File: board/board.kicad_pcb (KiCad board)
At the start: 4 copper layers, 29 x 29 mm, 32 parts, among them J1 001_I2C, J2 011_GPIO, Q1 Q_PMOS_DGS, Q2 Q_NMOS_DGS, U1 ALED7709ATR

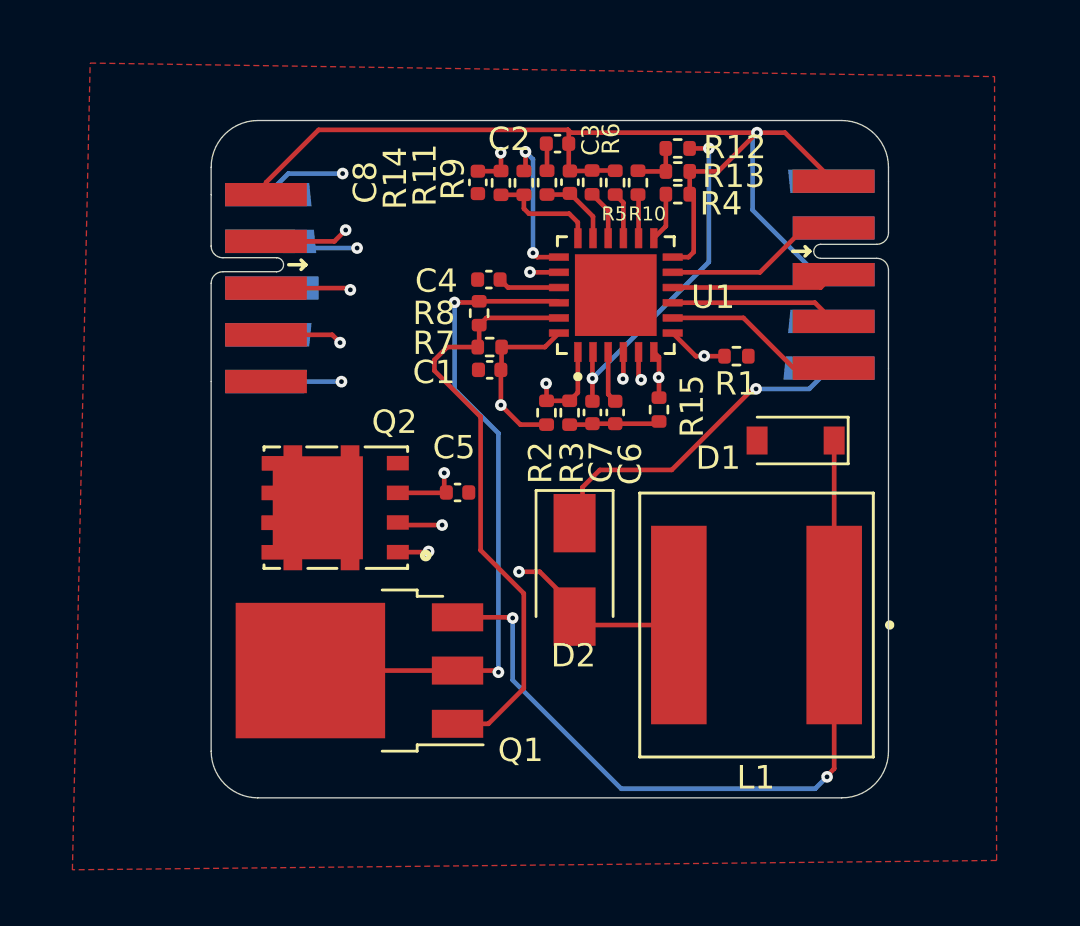
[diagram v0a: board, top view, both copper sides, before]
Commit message: Update PCB
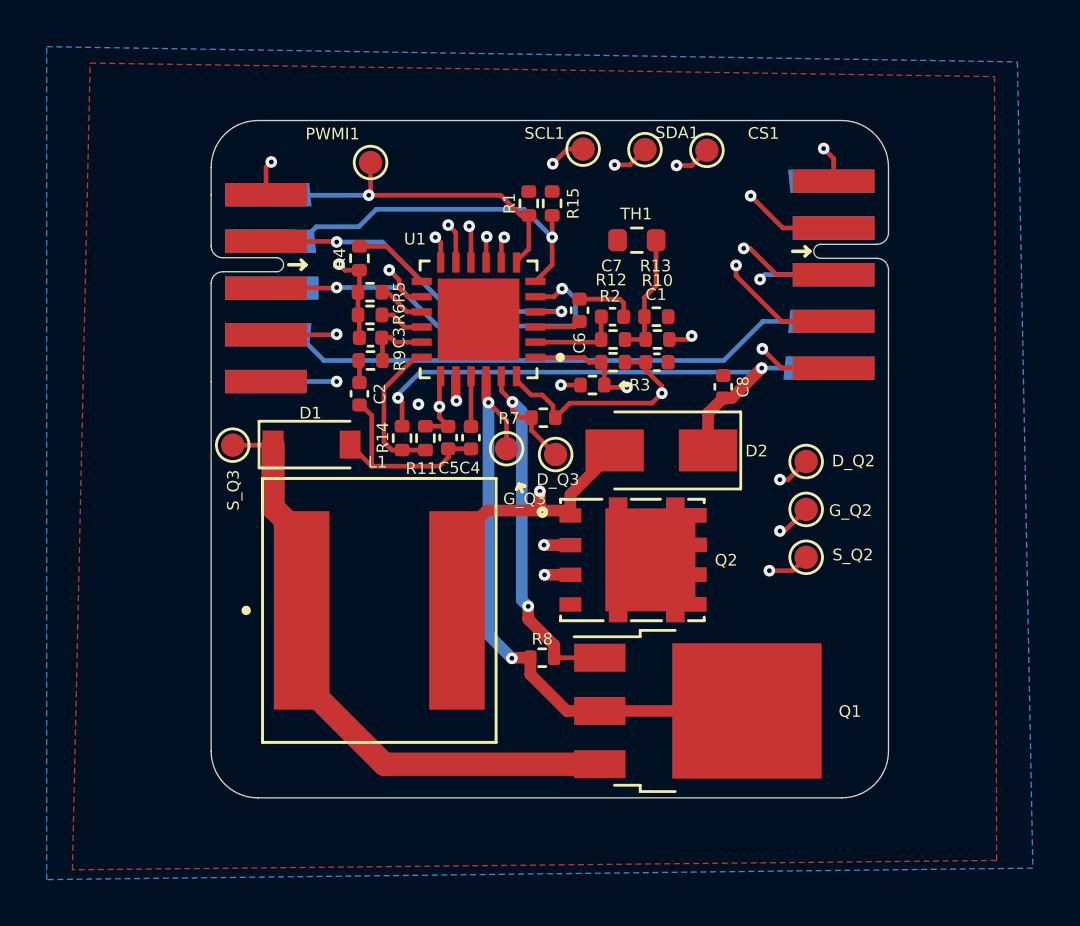
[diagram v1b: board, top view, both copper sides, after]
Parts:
- added CS1: TestPoint, TestPoint:TestPoint_Pad_D1.0mm, F.Cu at (161.2, 91.3)
- added D_Q2: TestPoint, TestPoint:TestPoint_Pad_D1.0mm, F.Cu at (165.5, 104.6)
- added D_Q3: TestPoint, TestPoint:TestPoint_Pad_D1.0mm, F.Cu at (154.8, 104.3)
- added G_Q2: TestPoint, TestPoint:TestPoint_Pad_D1.0mm, F.Cu at (165.5, 106.7)
- added G_Q3: TestPoint, TestPoint:TestPoint_Pad_D1.0mm, F.Cu at (152.7, 104.0)
- added PWMI1: TestPoint, TestPoint:TestPoint_Pad_D1.0mm, F.Cu at (146.8, 91.8)
- added SCL1: TestPoint, TestPoint:TestPoint_Pad_D1.0mm, F.Cu at (155.9, 91.2)
- added SDA1: TestPoint, TestPoint:TestPoint_Pad_D1.0mm, F.Cu at (158.6, 91.2)
- added S_Q2: TestPoint, TestPoint:TestPoint_Pad_D1.0mm, F.Cu at (165.5, 108.7)
- added S_Q3: TestPoint, TestPoint:TestPoint_Pad_D1.0mm, F.Cu at (140.9, 103.9)
- added TH1: 10kΩ, Resistor_SMD:R_0603_1608Metric, F.Cu at (158.2, 95.1)
- C1, C8: value C_Small -> 10uF
- C4, C6, C7: value C_Small -> 1uF
- L1: value L -> 15uH
- R10: value R_Small -> 2kΩ
- R12: value R_Small -> 1,8kΩ
- R13: value R_Small -> 1.1kΩ
- R4: value R_Small -> 6,8kΩ
- R5: value R_Small -> 62kΩ
- R7: value R_Small -> 39 mΩ
- moved D1 20.7 mm to (144.3, 103.9), turned to 0 degrees
- moved L1 16.2 mm to (147.2, 111.0), turned to 0 degrees
- moved R8 15.0 mm to (154.2, 113.0), turned to 0 degrees
- moved Q1 14.6 mm to (160.8, 115.3), turned to 0 degrees
- moved R4 13.9 mm to (146.3, 95.9), turned to 90 degrees
- moved C8 13.7 mm to (161.9, 101.4), turned to 90 degrees
- moved C2 13.7 mm to (146.3, 101.7), turned to -90 degrees
- moved Q2 12.9 mm to (158.0, 108.8), turned to 0 degrees
- moved R14 11.7 mm to (148.2, 103.6)
- moved R11 11.7 mm to (149.2, 103.6)
- moved R5 11.5 mm to (146.8, 97.3), turned to 0 degrees
- moved R6 11.1 mm to (146.8, 98.3), turned to 0 degrees
- moved R1 11.0 mm to (153.6, 93.5), turned to -90 degrees
- moved C3 10.8 mm to (146.8, 99.3), turned to 180 degrees
- moved R9 10.7 mm to (146.8, 100.3), turned to 0 degrees
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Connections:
- J1 pad 9: unconnected-(J1-3.3V-Pad9) -> 3.3V
- J2 pad 9: unconnected-(J2-3.3V-Pad9) -> 3.3V
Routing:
- net GND: track 50.4 -> 23.8 mm, vias 1 -> 7
- net 3.3V: track 0.00 -> 25.3 mm
- net /implementation/PWMI: track 34.5 -> 15.2 mm, vias 2 -> 1
- net /implementation/Enable: track 17.0 -> 33.3 mm, vias 2 -> 3
- net Net-(U1-TSNS): track 1.88 -> 18.0 mm, vias 0 -> 2
- net /implementation/common_Anode: track 37.8 -> 25.1 mm
- net /implementation/CH4: track 7.68 -> 19.9 mm, vias 0 -> 2
- net /implementation/CH3: track 7.12 -> 19.0 mm, vias 0 -> 2
- net Net-(D2-A): track 13.3 -> 24.8 mm
- net /implementation/CH2: track 7.22 -> 18.6 mm, vias 0 -> 2
- net Net-(U1-LDO3V3): track 14.9 -> 3.84 mm, vias 2 -> 0
- net /implementation/VIN: track 18.0 -> 27.8 mm
- net /implementation/CH1: track 7.78 -> 17.6 mm, vias 0 -> 2
- net Net-(D1-K): track 35.4 -> 26.6 mm, vias 2 -> 0
- net Net-(Q1-D): track 25.7 -> 18.2 mm, vias 0 -> 2
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- added copper zone on B.Cu, net GND
- added copper zone on In1.Cu, net GND
- added copper zone on In2.Cu, net GND
